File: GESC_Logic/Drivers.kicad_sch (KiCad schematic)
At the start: 27 parts, among them J3 gates_A, J4 gates_B, J5 gates_C, U4 INA241, U5 INA241, U6 INA241, U7 L6498DTR, U8 L6498DTR, U9 L6498DTR

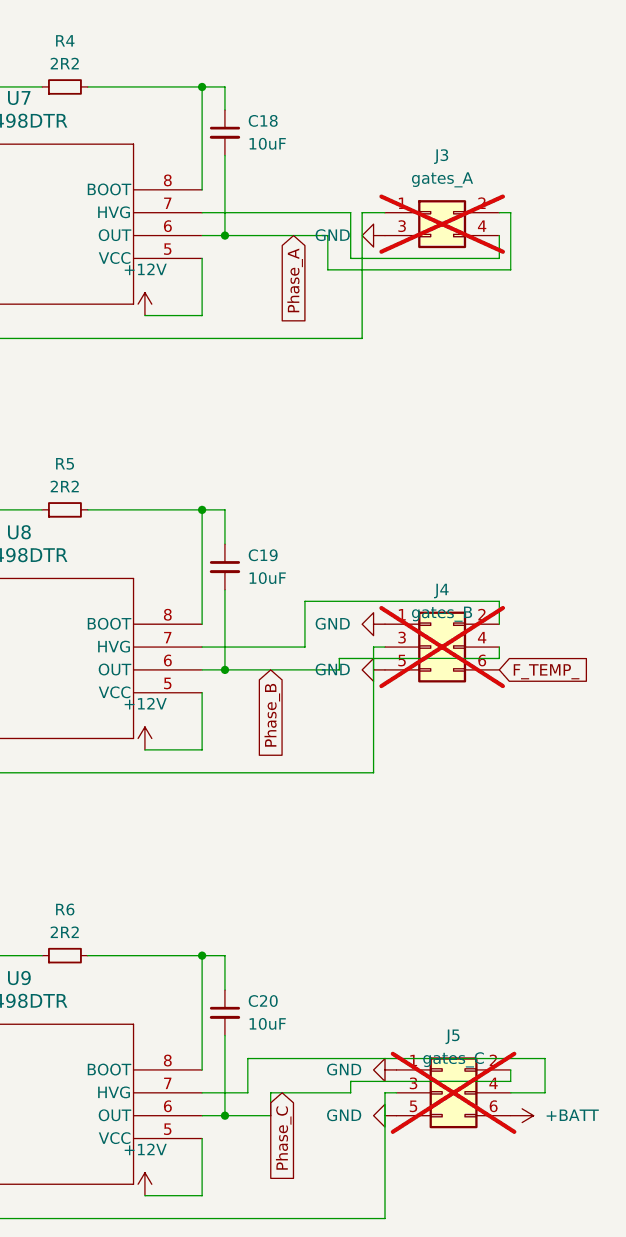
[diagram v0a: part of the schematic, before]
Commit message: asdf
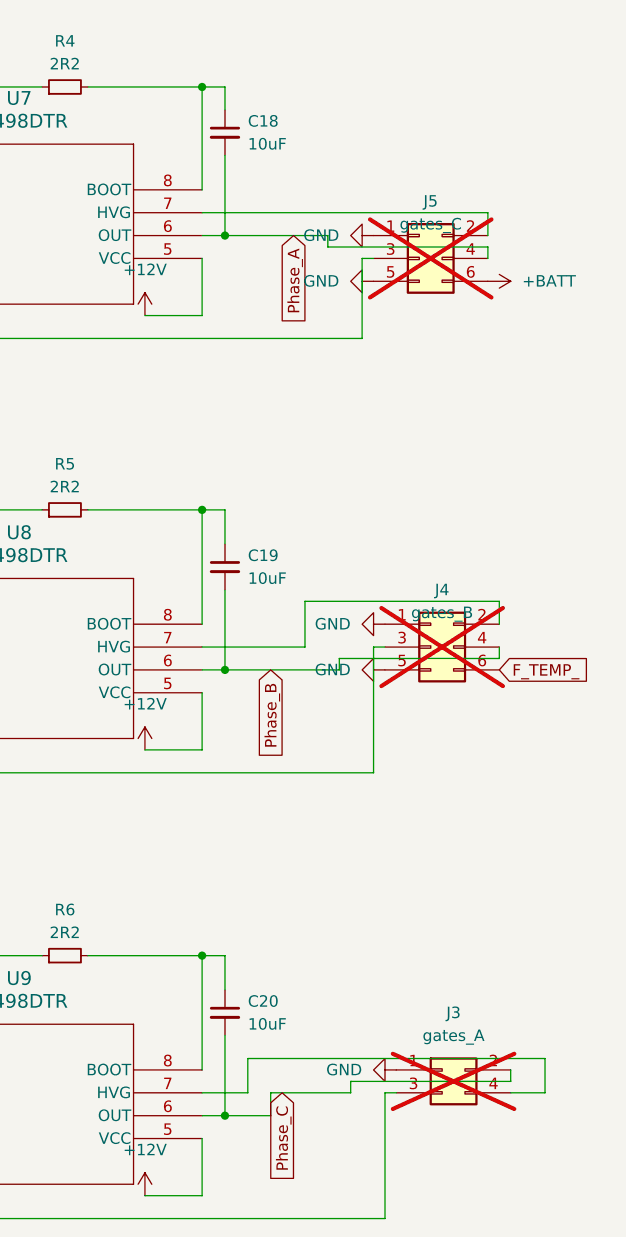
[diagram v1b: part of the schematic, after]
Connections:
- net GND: now also J3.1 (Pin_1); no longer J3.3 (Pin_3)
- net Phase_A: now also J5.4 (Pin_4); no longer J3.2 (Pin_2)
- net Phase_C: now also J3.2 (Pin_2); no longer J5.2 (Pin_2)
- net at U7.4 (LVG): now also J5.3 (Pin_3); no longer J3.1 (Pin_1)
- net at J3.4 (Pin_4): now also U9.7 (HVG); no longer U7.7 (HVG)
- net at U9.4 (LVG): now also J3.3 (Pin_3); no longer J5.3 (Pin_3)
- new net: J5.2 (Pin_2), U7.7 (HVG)
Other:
- moved on the sheet: J3, J5
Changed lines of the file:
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@@
 	(wire
 		(pts
-			(xy 186.69 50.8) (xy 186.69 64.77)
-		)
-		(stroke
-			(width 0)
-			(type default)
-		)
-	)
-	(wire
-		(pts
 			(xy 78.74 121.92) (xy 85.09 121.92)
 		)
@@
 	(wire
 		(pts
-			(xy 60.96 83.82) (xy 55.88 83.82)
+			(xy 168.91 50.8) (xy 200.66 50.8)
 		)
 		(stroke
@@
 	(wire
 		(pts
-			(xy 124.46 162.56) (xy 189.23 162.56)
-		)
-		(stroke
-			(width 0)
-			(type default)
-		)
-	)
-	(wire
-		(pts
-			(xy 189.23 50.8) (xy 186.69 50.8)
+			(xy 60.96 83.82) (xy 55.88 83.82)
 		)
 		(stroke
@@
 	(wire
 		(pts
-			(xy 185.42 50.8) (xy 185.42 55.88)
+			(xy 124.46 162.56) (xy 189.23 162.56)
 		)
 		(stroke
@@
 	(wire
 		(pts
-			(xy 190.5 148.59) (xy 189.23 148.59)
+			(xy 186.69 55.88) (xy 186.69 64.77)
 		)
 		(stroke
@@
 	(wire
 		(pts
-			(xy 185.42 55.88) (xy 201.93 55.88)
-		)
-		(stroke
-			(width 0)
-			(type default)
-		)
-	)
-	(wire
-		(pts
-			(xy 168.91 50.8) (xy 185.42 50.8)
-		)
-		(stroke
-			(width 0)
-			(type default)
-		)
-	)
-	(wire
-		(pts
 			(xy 171.45 53.34) (xy 182.88 53.34)
 		)
@@
 	(wire
 		(pts
+			(xy 189.23 148.59) (xy 190.5 148.59)
+		)
+		(stroke
+			(width 0)
+			(type default)
+		)
+	)
+	(wire
+		(pts
 			(xy 168.91 83.82) (xy 171.45 83.82)
 		)
@@
 	(wire
 		(pts
-			(xy 203.2 57.15) (xy 182.88 57.15)
+			(xy 200.66 55.88) (xy 200.66 54.61)
 		)
 		(stroke
@@
 	(wire
 		(pts
+			(xy 200.66 54.61) (xy 182.88 54.61)
+		)
+		(stroke
+			(width 0)
+			(type default)
+		)
+	)
+	(wire
+		(pts
 			(xy 185.42 148.59) (xy 185.42 147.32)
 		)
@@
 	(wire
 		(pts
-			(xy 168.91 133.35) (xy 171.45 133.35)
+			(xy 203.2 146.05) (xy 203.2 147.32)
 		)
 		(stroke
@@
 	(wire
 		(pts
-			(xy 201.93 55.88) (xy 201.93 53.34)
+			(xy 168.91 133.35) (xy 171.45 133.35)
 		)
 		(stroke
@@
 	(wire
 		(pts
-			(xy 182.88 53.34) (xy 182.88 57.15)
+			(xy 182.88 53.34) (xy 182.88 54.61)
 		)
 		(stroke
@@
 	(wire
 		(pts
-			(xy 201.93 50.8) (xy 203.2 50.8)
+			(xy 58.42 71.12) (xy 58.42 73.66)
 		)
 		(stroke
@@
 	(wire
 		(pts
-			(xy 58.42 71.12) (xy 58.42 73.66)
+			(xy 200.66 53.34) (xy 200.66 50.8)
 		)
 		(stroke
@@
 	(wire
 		(pts
-			(xy 171.45 142.24) (xy 171.45 151.13)
+			(xy 187.96 55.88) (xy 186.69 55.88)
 		)
 		(stroke
@@
 	(wire
 		(pts
-			(xy 203.2 148.59) (xy 207.01 148.59)
+			(xy 171.45 142.24) (xy 171.45 151.13)
 		)
 		(stroke
@@
 	(wire
 		(pts
-			(xy 203.2 50.8) (xy 203.2 57.15)
+			(xy 180.34 93.98) (xy 180.34 99.06)
 		)
 		(stroke
@@
 	(wire
 		(pts
-			(xy 180.34 93.98) (xy 180.34 99.06)
+			(xy 203.2 148.59) (xy 207.01 148.59)
 		)
 		(stroke
@@
 	(wire
 		(pts
-			(xy 203.2 147.32) (xy 203.2 146.05)
-		)
-		(stroke
-			(width 0)
-			(type default)
-		)
-	)
-	(wire
-		(pts
 			(xy 66.04 121.92) (xy 78.74 121.92)
 		)
@@
 	(symbol
 		(lib_id "power:GND")
-		(at 190.5 151.13 270)
+		(at 187.96 58.42 270)
 		(unit 1)
 		(exclude_from_sim no)
@@
 		(on_board yes)
 		(dnp no)
-		(fields_autoplaced yes)
 		(property "Reference" "#PWR042"
-			(at 184.15 151.13 0)
+			(at 181.61 58.42 0)
 			(effects
 				(font
@@
 		)
 		(property "Value" "GND"
-			(at 186.69 151.1299 90)
+			(at 184.15 58.4199 90)
 			(effects
 				(font
@@
 		)
 		(property "Footprint" ""
-			(at 190.5 151.13 0)
+			(at 187.96 58.42 0)
 			(effects
 				(font
@@
 		)
 		(property "Datasheet" ""
-			(at 190.5 151.13 0)
+			(at 187.96 58.42 0)
 			(effects
 				(font
@@
 		)
 		(property "Description" "Power symbol creates a global label with name \"GND\" , ground"
-			(at 190.5 151.13 0)
+			(at 187.96 58.42 0)
 			(effects
 				(font
@@
 	(symbol
 		(lib_id "Connector_Generic:Conn_02x02_Odd_Even")
-		(at 194.31 50.8 0)
+		(at 195.58 146.05 0)
 		(unit 1)
 		(exclude_from_sim no)
@@
 		(dnp yes)
 		(property "Reference" "J3"
-			(at 195.58 44.45 0)
+			(at 196.85 139.7 0)
 			(effects
 				(font
@@
 		)
 		(property "Value" "gates_A"
-			(at 195.58 46.99 0)
+			(at 196.85 142.24 0)
 			(effects
 				(font
@@
 		)
 		(property "Footprint" "Connector_PinHeader_2.00mm:PinHeader_2x02_P2.00mm_Vertical_SMD"
-			(at 194.31 50.8 0)
+			(at 195.58 146.05 0)
 			(effects
 				(font
@@
 		)
 		(property "Datasheet" "~"
-			(at 194.31 50.8 0)
+			(at 195.58 146.05 0)
 			(effects
 				(font
@@
 		)
 		(property "Description" "Generic connector, double row, 02x02, odd/even pin numbering scheme (row 1 odd numbers, row 2 even numbers), script generated (kicad-library-utils/schlib/autogen/connector/)"
-			(at 194.31 50.8 0)
+			(at 195.58 146.05 0)
 			(effects
 				(font
@@
 	(symbol
 		(lib_id "Connector_Generic:Conn_02x03_Odd_Even")
-		(at 195.58 148.59 0)
+		(at 193.04 55.88 0)
 		(unit 1)
 		(exclude_from_sim no)
@@
 		(dnp yes)
 		(property "Reference" "J5"
-			(at 196.85 142.24 0)
+			(at 194.31 49.53 0)
 			(effects
 				(font
@@
 		)
 		(property "Value" "gates_C"
-			(at 196.85 144.78 0)
+			(at 194.31 52.07 0)
 			(effects
 				(font
@@
 		)
 		(property "Footprint" "Connector_PinSocket_2.00mm:PinSocket_2x03_P2.00mm_Vertical_SMD"
-			(at 195.58 148.59 0)
+			(at 193.04 55.88 0)
 			(effects
 				(font
@@
 		)
 		(property "Datasheet" "~"
-			(at 195.58 148.59 0)
+			(at 193.04 55.88 0)
 			(effects
 				(font
@@
 		)
 		(property "Description" "Generic connector, double row, 02x03, odd/even pin numbering scheme (row 1 odd numbers, row 2 even numbers), script generated (kicad-library-utils/schlib/autogen/connector/)"
-			(at 195.58 148.59 0)
+			(at 193.04 55.88 0)
 			(effects
 				(font
@@
 	(symbol
 		(lib_id "power:GND")
-		(at 189.23 53.34 270)
+		(at 187.96 53.34 270)
 		(unit 1)
 		(exclude_from_sim no)
@@
 		(dnp no)
 		(property "Reference" "#PWR039"
-			(at 182.88 53.34 0)
+			(at 181.61 53.34 0)
 			(effects
 				(font
@@
 		)
 		(property "Value" "GND"
-			(at 185.42 53.3399 90)
+			(at 184.15 53.3399 90)
 			(effects
 				(font
@@
 		)
 		(property "Footprint" ""
-			(at 189.23 53.34 0)
+			(at 187.96 53.34 0)
 			(effects
 				(font
@@
 		)
 		(property "Datasheet" ""
-			(at 189.23 53.34 0)
+			(at 187.96 53.34 0)
 			(effects
 				(font
@@
 		)
 		(property "Description" "Power symbol creates a global label with name \"GND\" , ground"
-			(at 189.23 53.34 0)
+			(at 187.96 53.34 0)
 			(effects
 				(font
@@
 	(symbol
 		(lib_id "power:+BATT")
-		(at 203.2 151.13 270)
+		(at 200.66 58.42 270)
 		(unit 1)
 		(exclude_from_sim no)
@@
 		(fields_autoplaced yes)
 		(property "Reference" "#PWR038"
-			(at 199.39 151.13 0)
+			(at 196.85 58.42 0)
 			(effects
 				(font
@@
 		)
 		(property "Value" "+BATT"
-			(at 207.01 151.1299 90)
+			(at 204.47 58.4199 90)
 			(effects
 				(font
@@
 		)
 		(property "Footprint" ""
-			(at 203.2 151.13 0)
+			(at 200.66 58.42 0)
 			(effects
 				(font
@@
 		)
 		(property "Datasheet" ""
-			(at 203.2 151.13 0)
+			(at 200.66 58.42 0)
 			(effects
 				(font
@@
 		)
 		(property "Description" "Power symbol creates a global label with name \"+BATT\""
-			(at 203.2 151.13 0)
+			(at 200.66 58.42 0)
 			(effects
 				(font
